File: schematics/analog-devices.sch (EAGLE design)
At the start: 22 parts, among them IC1 TLC271D, IC2 TLC271D

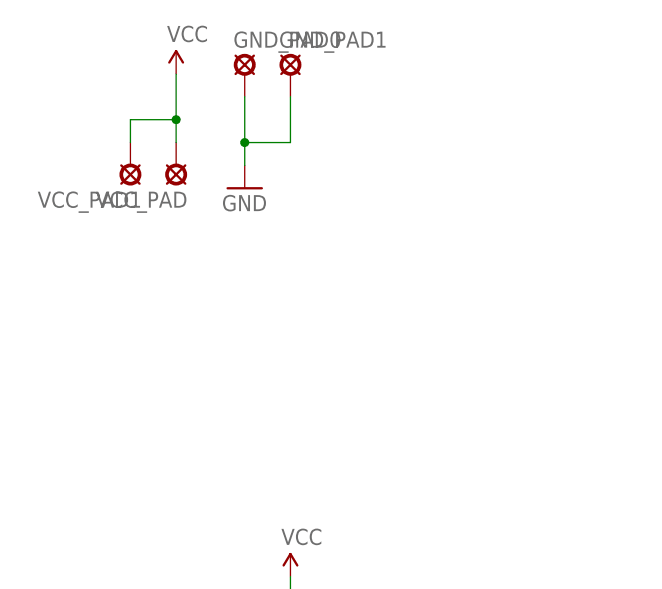
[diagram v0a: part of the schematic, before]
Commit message: Платы, правки, накопленные изменения
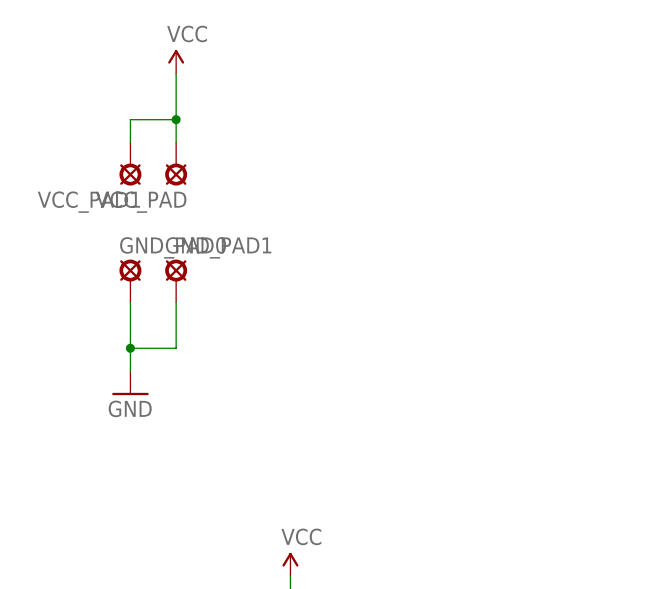
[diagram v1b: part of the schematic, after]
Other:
- moved on the sheet: GND_PAD0, GND_PAD1
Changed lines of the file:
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@@
 <instance part="O2_PAD" gate="1" x="198.12" y="58.42" rot="R270"/>
 <instance part="CO2_PAD" gate="1" x="200.66" y="0" rot="R270"/>
-<instance part="GND_PAD0" gate="1" x="25.4" y="83.82"/>
+<instance part="GND_PAD0" gate="1" x="12.7" y="60.96"/>
 <instance part="SUPPLY1" gate="G$1" x="17.78" y="83.82"/>
-<instance part="GND1" gate="1" x="25.4" y="71.12"/>
+<instance part="GND1" gate="1" x="12.7" y="48.26"/>
 <instance part="GND2" gate="1" x="86.36" y="-17.78"/>
 <instance part="SUPPLY2" gate="G$1" x="86.36" y="7.62"/>
@@
 <instance part="R5" gate="G$1" x="162.56" y="-27.94" rot="R180"/>
 <instance part="GND6" gate="1" x="137.16" y="-33.02"/>
-<instance part="GND_PAD1" gate="1" x="30.48" y="83.82"/>
+<instance part="GND_PAD1" gate="1" x="17.78" y="60.96"/>
 <instance part="GND11" gate="1" x="119.38" y="35.56"/>
 <instance part="VCC_PAD1" gate="1" x="12.7" y="73.66" rot="R180"/>
@@
 <pinref part="GND_PAD0" gate="1" pin="MP"/>
 <pinref part="GND1" gate="1" pin="GND"/>
-<wire x1="25.4" y1="81.28" x2="25.4" y2="76.2" width="0.1524" layer="91"/>
+<wire x1="12.7" y1="58.42" x2="12.7" y2="53.34" width="0.1524" layer="91"/>
 <pinref part="GND_PAD1" gate="1" pin="MP"/>
-<wire x1="25.4" y1="76.2" x2="25.4" y2="73.66" width="0.1524" layer="91"/>
-<wire x1="25.4" y1="76.2" x2="30.48" y2="76.2" width="0.1524" layer="91"/>
-<wire x1="30.48" y1="76.2" x2="30.48" y2="81.28" width="0.1524" layer="91"/>
-<junction x="25.4" y="76.2"/>
+<wire x1="12.7" y1="53.34" x2="12.7" y2="50.8" width="0.1524" layer="91"/>
+<wire x1="12.7" y1="53.34" x2="17.78" y2="53.34" width="0.1524" layer="91"/>
+<wire x1="17.78" y1="53.34" x2="17.78" y2="58.42" width="0.1524" layer="91"/>
+<junction x="12.7" y="53.34"/>
 </segment>
 <segment>
